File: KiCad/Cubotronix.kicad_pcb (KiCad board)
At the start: 2 copper layers, 35 x 35 mm, 32 parts, among them J1 Vin, J2 ADC, J3 GPIO12, J4 GPIO15, P2 Battery, P5 USB-Serial, P6 I2C/1-W, SW1 Boot, SW2 Reset, U1 AP2114H-3.3TRG1, U2 MCP73831T-2ATI/OT, U3 ESP-12E

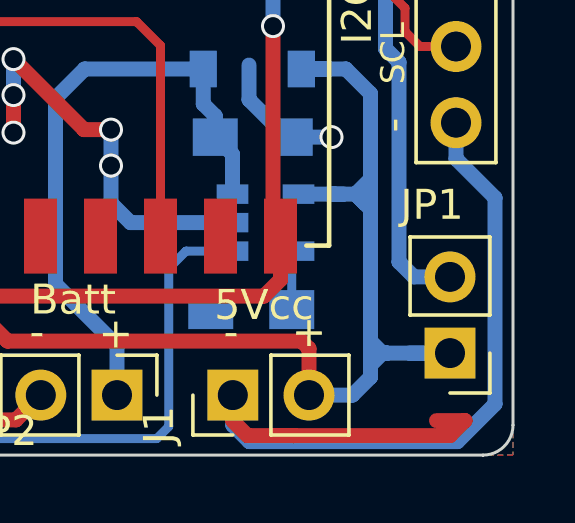
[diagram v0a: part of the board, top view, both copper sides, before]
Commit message: change on/off pin
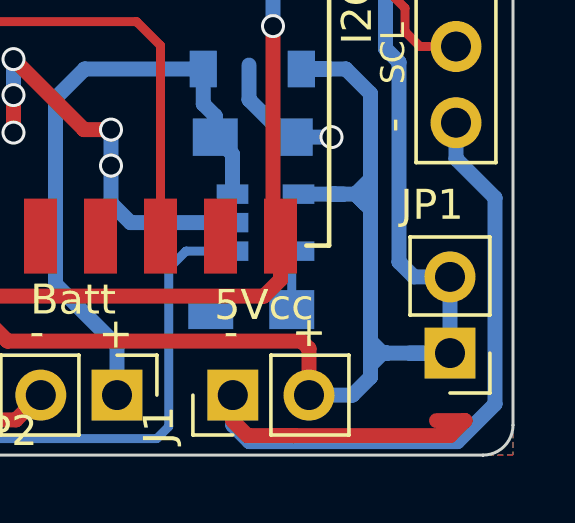
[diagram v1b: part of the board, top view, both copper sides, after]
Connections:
- C1 pad 1: Net-(C1-Pad1) -> VCC
- JP1 pad 2: Net-(C1-Pad1) -> VCC
- U1 pad 3: Net-(C1-Pad1) -> VCC
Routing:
- net VCC: track 69.0 -> 98.7 mm
- net Net-(C1-Pad1): track 27.1 -> 0.00 mm
- net (no net): track 0.00 -> 4.60 mm, vias 0 -> 4
- net GND: track 84.7 -> 80.1 mm, vias 16 -> 12
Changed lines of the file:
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@@
 (kicad_pcb (version 4) (host pcbnew 4.0.7)
   (general
-    (links 65)
-    (no_connects 0)
+    (links 66)
+    (no_connects 2)
     (area 114.949999 54.949999 150.050001 90.050001)
     (thickness 1.6)
     (drawings 24)
-    (tracks 362)
+    (tracks 363)
     (zones 0)
     (modules 32)
-    (nets 28)
+    (nets 27)
   )
   (page A4)
@@
   (net 25 /GPIO14)
   (net 26 /GPIO13)
-  (net 27 "Net-(C1-Pad1)")
   (net_class Default "Esta es la clase de red por defecto."
     (clearance 0.2)
@@
     (add_net /TX)
     (add_net GND)
-    (add_net "Net-(C1-Pad1)")
     (add_net VCC)
   )
@@
     (fp_line (start -0.5 -0.85) (end 0.5 -0.85) (layer B.SilkS) (width 0.15))
     (pad 1 smd rect (at -1.25 0 270) (size 1.5 1.25) (layers B.Cu B.Paste B.Mask)
-      (net 27 "Net-(C1-Pad1)"))
+      (net 1 VCC))
     (pad 2 smd rect (at 1.25 0 270) (size 1.5 1.25) (layers B.Cu B.Paste B.Mask)
       (net 2 GND))
@@
       (net 1 VCC))
     (pad 2 thru_hole oval (at 0 2.54 180) (size 1.7 1.7) (drill 1) (layers *.Cu *.Mask)
-      (net 27 "Net-(C1-Pad1)"))
+      (net 1 VCC))
     (model ${KISYS3DMOD}/Pin_Headers.3dshapes/Pin_Header_Straight_1x02_Pitch2.54mm.wrl
       (at (xyz 0 0 0))
@@
       (net 3 +3V3))
     (pad 3 smd rect (at -3.15 -2.3 90) (size 2 1.5) (layers B.Cu B.Paste B.Mask)
-      (net 27 "Net-(C1-Pad1)"))
+      (net 1 VCC))
     (pad 1 smd rect (at -3.15 2.3 90) (size 2 1.5) (layers B.Cu B.Paste B.Mask)
       (net 2 GND))
@@
     (arrow2b (pts (xy 115 95) (xy 116.126504 94.413579)))
   )
+  (segment (start 137.75 72.75) (end 136.5 72.75) (width 0.5) (layer F.Cu) (net 0))
+  (via (at 136.5 72.75) (size 0.8) (drill 0.6) (layers F.Cu B.Cu) (net 0))
+  (segment (start 139 72.75) (end 137.75 72.75) (width 0.5) (layer B.Cu) (net 0))
+  (via (at 137.75 72.75) (size 0.8) (drill 0.6) (layers F.Cu B.Cu) (net 0))
+  (segment (start 140.15 72.75) (end 139 72.75) (width 0.5) (layer F.Cu) (net 0))
+  (via (at 139 72.75) (size 0.8) (drill 0.6) (layers F.Cu B.Cu) (net 0))
+  (segment (start 140.75 73.45) (end 140.15 72.85) (width 0.5) (layer B.Cu) (net 0))
+  (segment (start 140.15 72.85) (end 140.15 72.75) (width 0.5) (layer B.Cu) (net 0))
+  (via (at 140.15 72.75) (size 0.8) (drill 0.6) (layers F.Cu B.Cu) (net 0))
+  (segment (start 147.9 84.06) (end 147.9 86.6) (width 0.5) (layer B.Cu) (net 1))
   (segment (start 142.95 86.2) (end 143.2 86.45) (width 0.5) (layer F.Cu) (net 1))
   (segment (start 142.95 86.2) (end 133.15 86.2) (width 0.5) (layer F.Cu) (net 1))
@@
   (segment (start 147.9 86.6) (end 146.55 86.6) (width 0.5) (layer B.Cu) (net 1))
   (segment (start 143.9 77.13) (end 142.945 77.13) (width 0.5) (layer B.Cu) (net 1))
+  (segment (start 147.9 84.06) (end 146.697919 84.06) (width 0.5) (layer B.Cu) (net 1))
+  (segment (start 146.2 83.562081) (end 146.2 76.9) (width 0.5) (layer B.Cu) (net 1))
+  (segment (start 146.2 76.9) (end 145.75 76.45) (width 0.5) (layer B.Cu) (net 1))
+  (segment (start 146.697919 84.06) (end 146.2 83.562081) (width 0.5) (layer B.Cu) (net 1))
+  (segment (start 145.75 76.45) (end 145.75 70.8) (width 0.5) (layer B.Cu) (net 1))
+  (segment (start 145.75 70.8) (end 145.25 70.3) (width 0.5) (layer B.Cu) (net 1))
+  (segment (start 145.25 70.3) (end 143.6 70.3) (width 0.5) (layer B.Cu) (net 1))
+  (segment (start 142.9 69.6) (end 142.9 66.9) (width 0.5) (layer B.Cu) (net 1))
+  (segment (start 143.6 70.3) (end 142.9 69.6) (width 0.5) (layer B.Cu) (net 1))
+  (segment (start 142.9 66.9) (end 142.9 63.45) (width 0.5) (layer B.Cu) (net 1))
+  (segment (start 142.9 63.45) (end 140.25 63.45) (width 0.5) (layer B.Cu) (net 1))
+  (segment (start 140.25 63.45) (end 140.2 63.4) (width 0.5) (layer B.Cu) (net 1))
+  (segment (start 142.95 63.5) (end 142.9 63.45) (width 0.3) (layer B.Cu) (net 1))
   (segment (start 148.1 78.92) (end 148.1 80.122081) (width 0.5) (layer B.Cu) (net 2))
   (segment (start 148.1 80.122081) (end 149.4 81.422081) (width 0.5) (layer B.Cu) (net 2))
@@
   (segment (start 140.2 70.25) (end 141.75 70.25) (width 0.5) (layer B.Cu) (net 2))
   (via (at 141.75 70.25) (size 0.8) (drill 0.6) (layers F.Cu B.Cu) (net 2))
-  (segment (start 137.75 72.75) (end 136.5 72.75) (width 0.5) (layer F.Cu) (net 2))
-  (via (at 136.5 72.75) (size 0.8) (drill 0.6) (layers F.Cu B.Cu) (net 2))
-  (segment (start 139 72.75) (end 137.75 72.75) (width 0.5) (layer B.Cu) (net 2))
-  (via (at 137.75 72.75) (size 0.8) (drill 0.6) (layers F.Cu B.Cu) (net 2))
-  (segment (start 140.15 72.75) (end 139 72.75) (width 0.5) (layer F.Cu) (net 2))
-  (via (at 139 72.75) (size 0.8) (drill 0.6) (layers F.Cu B.Cu) (net 2))
   (segment (start 142.7 89.35) (end 141.15 89.35) (width 0.5) (layer F.Cu) (net 2))
   (segment (start 140.66 88) (end 140.66 88.86) (width 0.5) (layer F.Cu) (net 2))
@@
   (segment (start 140.2 65.9) (end 140.2 70.25) (width 0.5) (layer B.Cu) (net 2))
   (via (at 140.2 70.25) (size 0.8) (drill 0.6) (layers F.Cu B.Cu) (net 2))
-  (segment (start 140.75 73.45) (end 140.15 72.85) (width 0.5) (layer B.Cu) (net 2))
-  (segment (start 140.15 72.85) (end 140.15 72.75) (width 0.5) (layer B.Cu) (net 2))
-  (via (at 140.15 72.75) (size 0.8) (drill 0.6) (layers F.Cu B.Cu) (net 2))
   (segment (start 142.575 79.4) (end 142.45 79.4) (width 0.5) (layer B.Cu) (net 2))
   (via (at 118.2 85) (size 0.8) (drill 0.6) (layers F.Cu B.Cu) (net 3))
@@
   (segment (start 138.7 65.25) (end 139 64.95) (width 0.3) (layer F.Cu) (net 23))
   (segment (start 139 64.95) (end 139 59.7) (width 0.3) (layer F.Cu) (net 23))
-  (segment (start 147.9 84.06) (end 146.697919 84.06) (width 0.5) (layer B.Cu) (net 27))
-  (segment (start 146.2 83.562081) (end 146.2 76.9) (width 0.5) (layer B.Cu) (net 27))
-  (segment (start 146.2 76.9) (end 145.75 76.45) (width 0.5) (layer B.Cu) (net 27))
-  (segment (start 146.697919 84.06) (end 146.2 83.562081) (width 0.5) (layer B.Cu) (net 27))
-  (segment (start 145.75 76.45) (end 145.75 70.8) (width 0.5) (layer B.Cu) (net 27))
-  (segment (start 145.75 70.8) (end 145.25 70.3) (width 0.5) (layer B.Cu) (net 27))
-  (segment (start 145.25 70.3) (end 143.6 70.3) (width 0.5) (layer B.Cu) (net 27))
-  (segment (start 142.9 69.6) (end 142.9 66.9) (width 0.5) (layer B.Cu) (net 27))
-  (segment (start 143.6 70.3) (end 142.9 69.6) (width 0.5) (layer B.Cu) (net 27))
-  (segment (start 142.9 66.9) (end 142.9 63.45) (width 0.5) (layer B.Cu) (net 27))
-  (segment (start 142.9 63.45) (end 140.25 63.45) (width 0.5) (layer B.Cu) (net 27))
-  (segment (start 140.25 63.45) (end 140.2 63.4) (width 0.5) (layer B.Cu) (net 27))
-  (segment (start 142.95 63.5) (end 142.9 63.45) (width 0.3) (layer B.Cu) (net 27))
   (zone (net 0) (net_name "") (layer F.Cu) (hatch edge 0.508)
     (connect_pads (clearance 0.508))
